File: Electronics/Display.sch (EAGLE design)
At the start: 14 parts, among them IC1 4081N, IC2 74HC165N, T1 BC547, T2 BC547, X4 HD44780LCD-1602

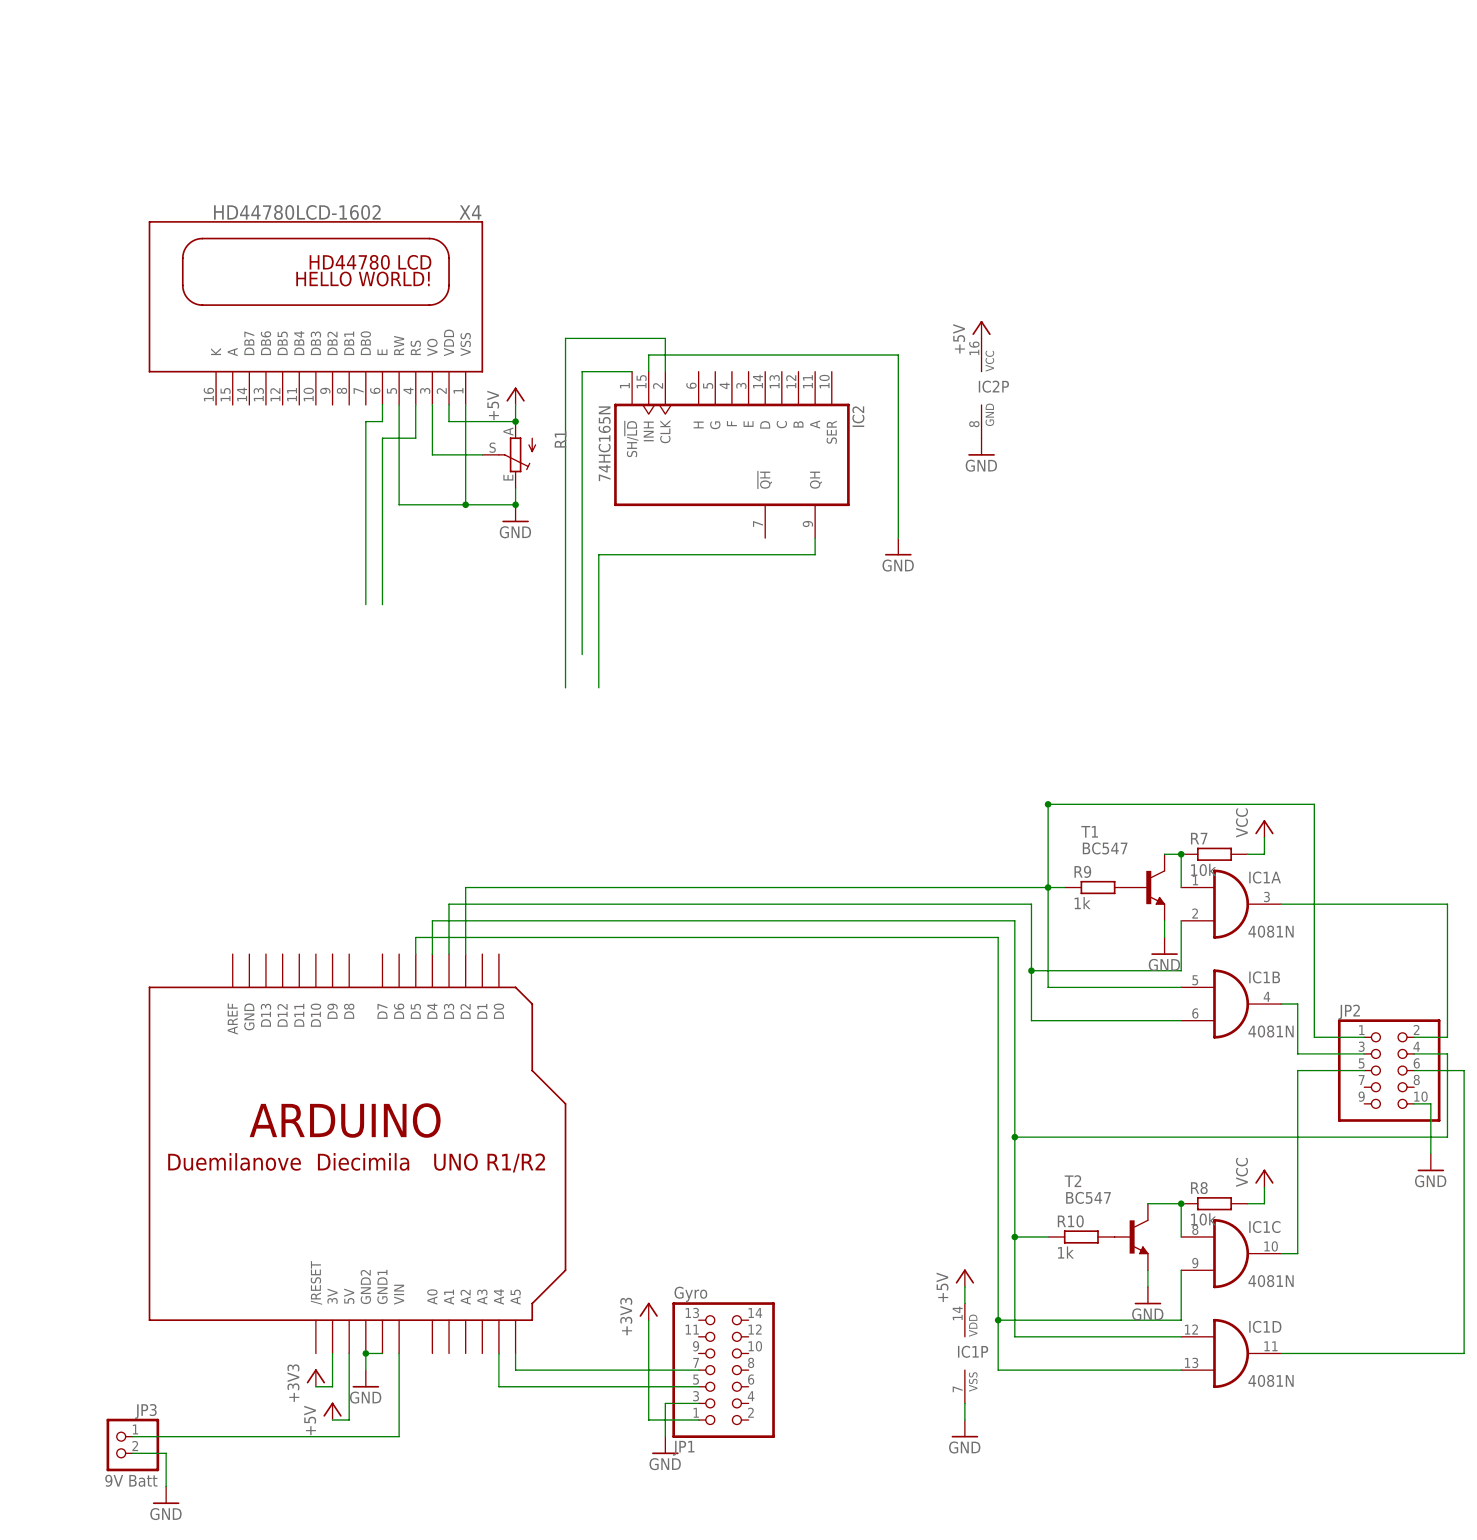
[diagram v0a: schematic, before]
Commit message: 
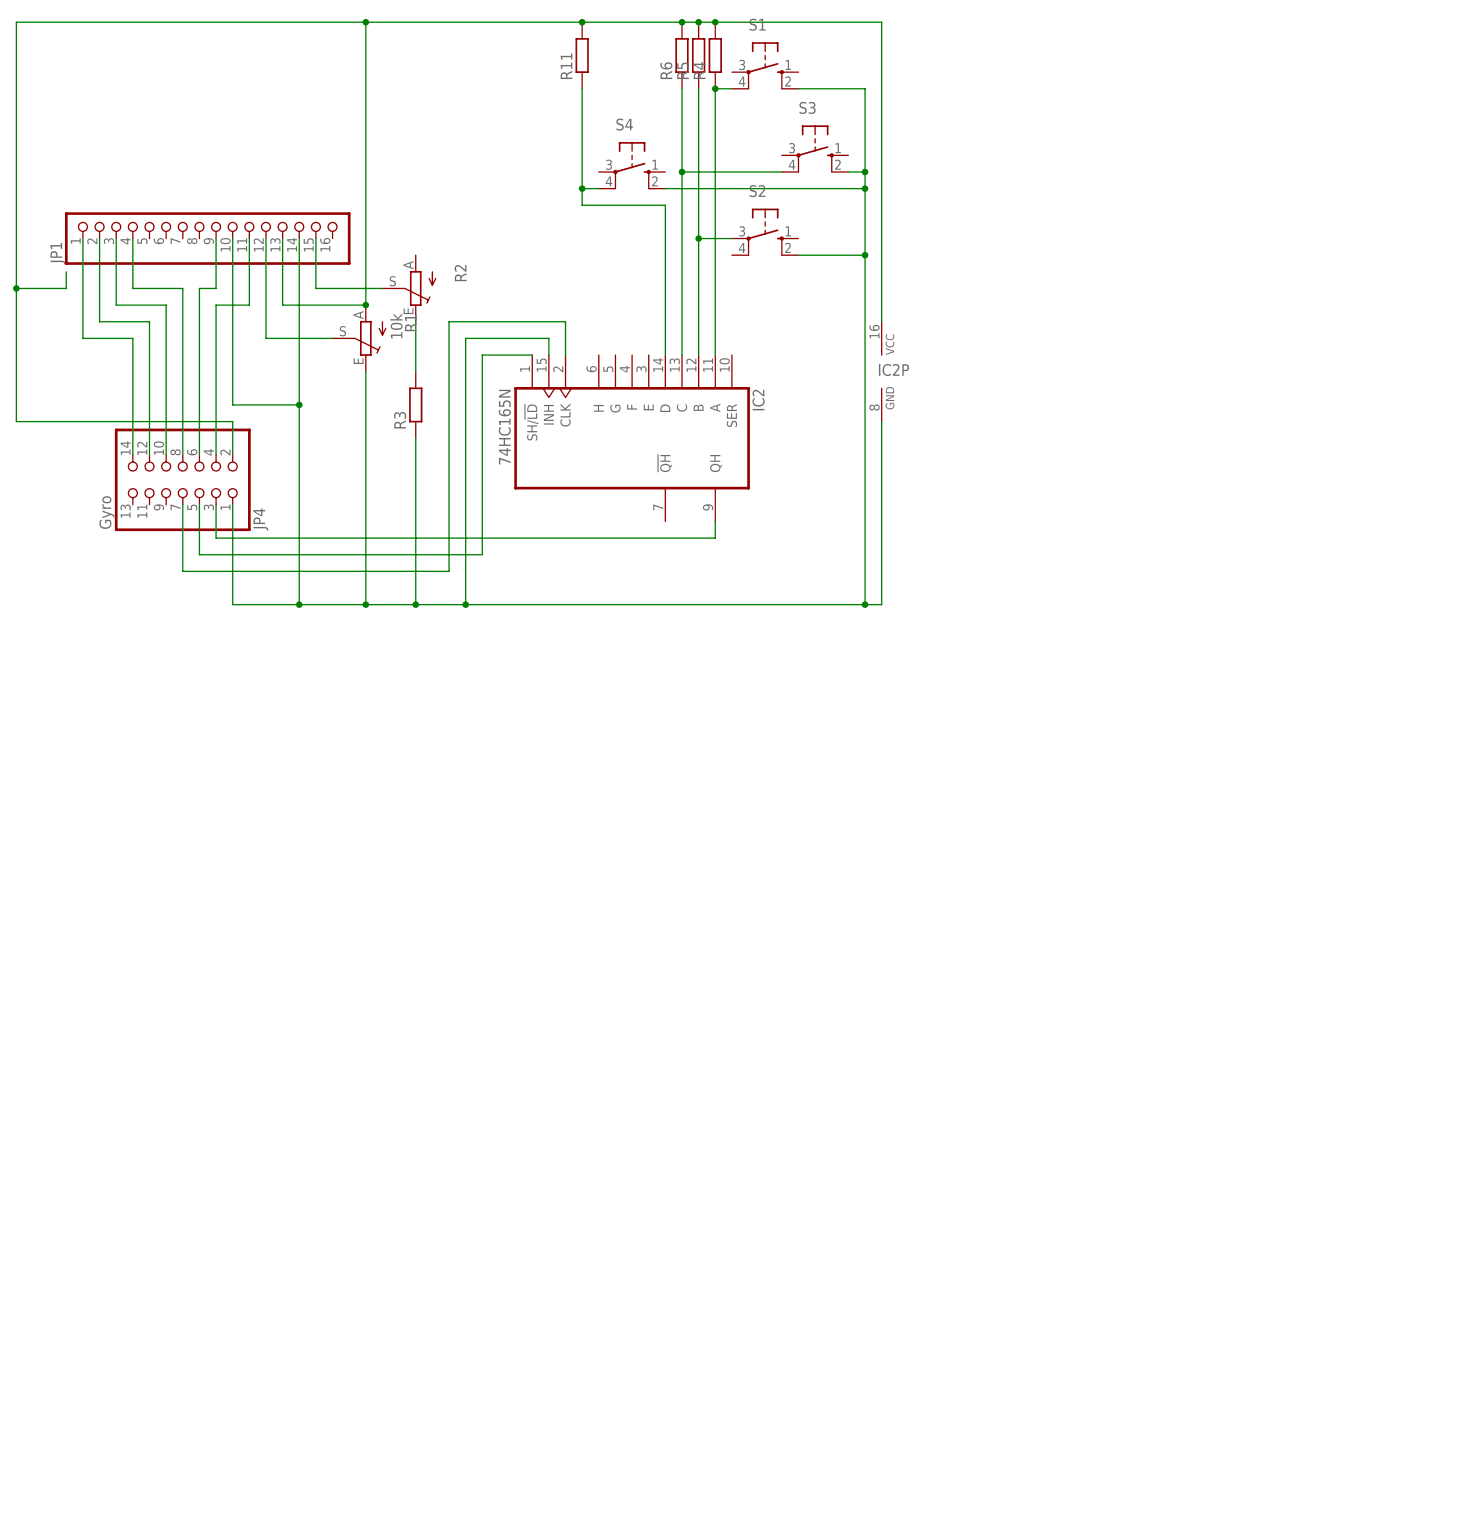
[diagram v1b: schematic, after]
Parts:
- removed IC1: 4081N, 40xx:4081N
- removed JP2: (no value), pinhead:PINHD-2X5
- removed JP3: 9V Batt, pinhead:PINHD-1X2
- removed R10, R9: 1k, rcl:R-EU_0207/10
- removed R7, R8: 10k, rcl:R-EU_0207/10
- removed T1, T2: BC547, transistor:BC547
- removed U$1: ARDUINOUNO, adafruit:ARDUINOUNO
- removed X4: HD44780LCD-1602, adafruit:HD44780LCD-1602
- added JP4: Gyro, pinhead:PINHD-2X7
- added R11, R3, R4, R5, R6: (no value), rcl:R-EU_0207/10
- added R2: (no value), pot:TRIM_EU-CA9H
- added S1, S2, S3, S4: (no value), switch-omron:10-XX
- JP1: value Gyro -> (none); device pinhead:PINHD-2X7 -> pinhead:PINHD-1X16
- R1: value (none) -> 10k
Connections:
- removed net +3V3: JP1.1, U$1.3V
- removed net +5V: IC2P.VCC, R1.A, X4.VDD
- removed net GND: IC1P.VSS, IC2A.INH, IC2P.GND, JP1.3, JP2.10, JP3.2, R1.E, T1.E, T2.E, U$1.GND1, U$1.GND2, X4.RW, X4.VSS
- removed net N$10: IC1B.I0, JP2.1, R9.1, U$1.D2
- removed net N$11: IC1A.I1, IC1B.I1, U$1.D3
- removed net N$16: IC1C.I0, R8.1, T2.C
- removed net N$17: R9.2, T1.B
- removed net N$20: R10.2, T2.B
- removed net N$26: JP1.7, U$1.A5
- removed net N$39: JP3.1, U$1.VIN
- removed net N$41: JP1.5, U$1.A4
- removed net N$5: IC1D.O, JP2.6
- removed net N$7: IC1C.I1, IC1D.I1, U$1.D5
- removed net N$8: IC1A.I0, R7.1, T1.C
- removed net VCC: IC1P.VDD, R7.2, R8.2, U$1.5V
- new net N$18: JP1.4, JP4.8
- new net N$19: JP1.3, JP4.10
- new net N$21: JP1.2, JP4.12
- new net N$22: JP1.1, JP4.14
- new net N$32: IC2A.A, R4.1, S1.P1
- new net N$34: IC2A.B, R5.1, S2.P
- new net N$35: IC2A.C, R6.1, S3.P1
- new net N$36: IC2A.D, R11.1, S4.P1
- net N$1: now also JP1.15, R2.S; no longer IC1A.O, JP2.2
- net N$12: now also JP1.12; no longer X4.VO
- net N$13: now also JP4.3
- net N$14: now also JP4.7
- net N$15: now also JP1.9, JP4.6; no longer X4.E
- net N$2: now also IC2A.INH, IC2P.GND, JP1.10, JP1.14, JP4.1, R1.E, R3.1, S1.S1, S2.S1, S3.S1, S4.S1; no longer IC1B.O, JP2.3
- net N$3: now also JP1.13, JP4.2, R1.A, R11.2, R4.2, R5.2, R6.2; no longer IC1D.I0, JP2.4, R10.1, U$1.D4
- net N$4: now also R2.E, R3.2; no longer IC1C.O, JP2.5
- net N$6: now also JP1.11, JP4.4; no longer X4.RS
- net N$9: now also JP4.5
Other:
- moved on the sheet: IC2, IC2P, R1
